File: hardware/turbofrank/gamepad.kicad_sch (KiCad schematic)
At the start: 3 parts, among them J7 D-SUB 9 Male

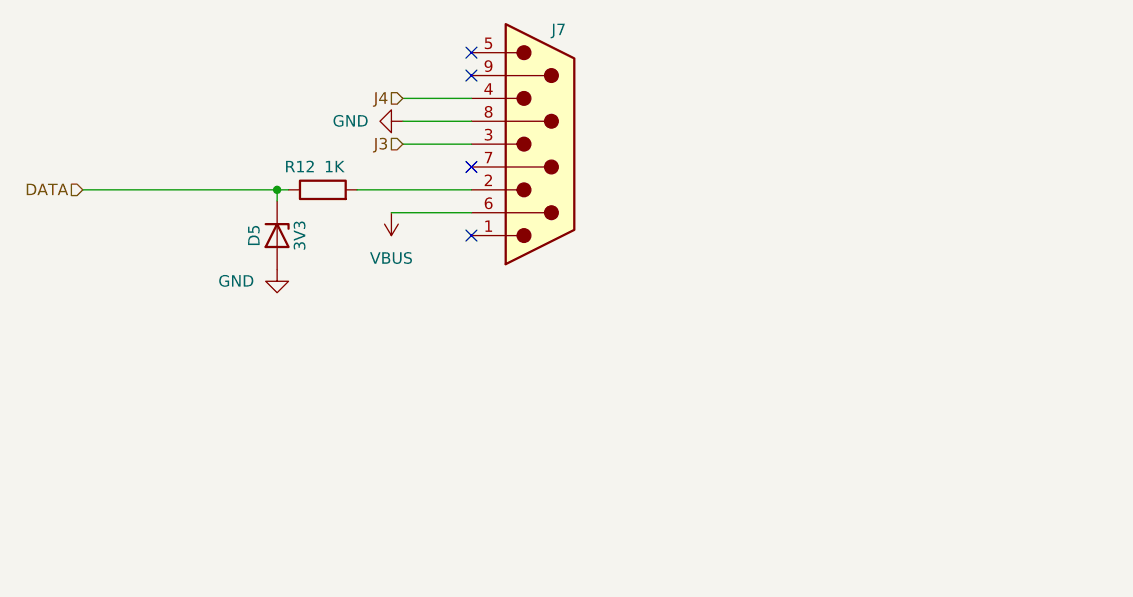
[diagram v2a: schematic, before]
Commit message: TurboFRANK HW 1.05 Release
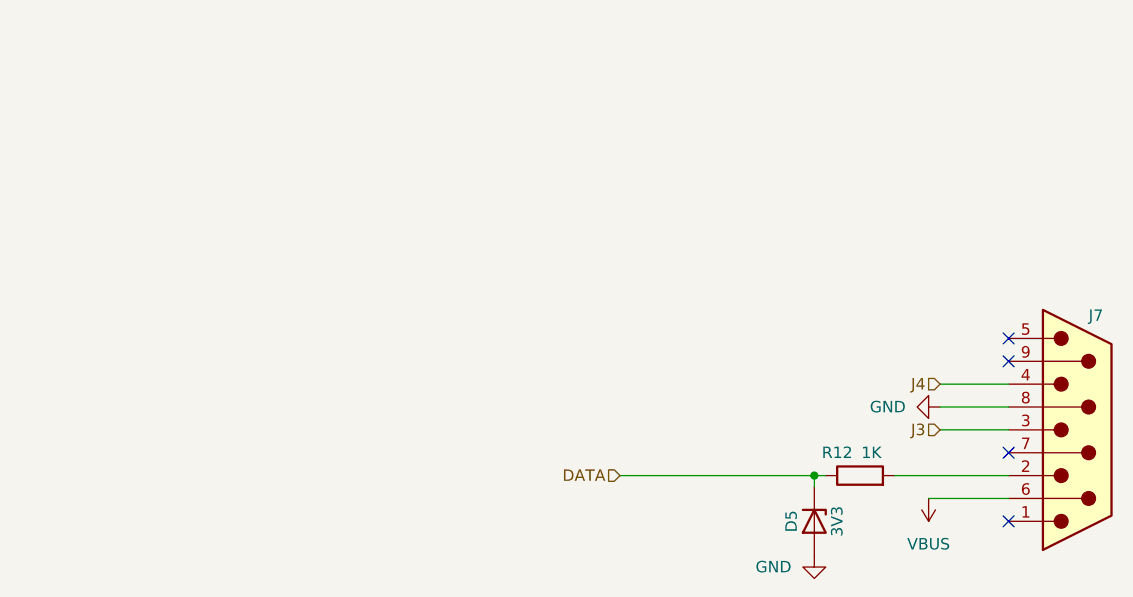
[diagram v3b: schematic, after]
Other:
- moved on the sheet: D5, J7, R12
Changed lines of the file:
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@@
 	)
 	(junction
-		(at 78.74 68.58)
+		(at 138.43 100.33)
 		(diameter 0)
 		(color 0 0 0 0)
 	)
 	(no_connect
-		(at 100.33 55.88)
+		(at 160.02 87.63)
 	)
 	(no_connect
-		(at 100.33 53.34)
+		(at 160.02 85.09)
 	)
 	(no_connect
-		(at 100.33 66.04)
+		(at 160.02 97.79)
 	)
 	(no_connect
-		(at 100.33 73.66)
-	)
-	(wire
-		(pts
-			(xy 92.71 63.5) (xy 100.33 63.5)
-		)
-		(stroke
-			(width 0)
-			(type default)
-		)
-	)
-	(wire
-		(pts
-			(xy 92.71 58.42) (xy 100.33 58.42)
-		)
-		(stroke
-			(width 0)
-			(type default)
-		)
-	)
-	(wire
-		(pts
-			(xy 91.44 71.12) (xy 100.33 71.12)
-		)
-		(stroke
-			(width 0)
-			(type default)
-		)
-	)
-	(wire
-		(pts
-			(xy 78.74 68.58) (xy 78.74 69.85)
-		)
-		(stroke
-			(width 0)
-			(type default)
-		)
-	)
-	(wire
-		(pts
-			(xy 57.15 68.58) (xy 78.74 68.58)
-		)
-		(stroke
-			(width 0)
-			(type default)
-		)
-	)
-	(wire
-		(pts
-			(xy 80.01 68.58) (xy 78.74 68.58)
-		)
-		(stroke
-			(width 0)
-			(type default)
-		)
-	)
-	(wire
-		(pts
-			(xy 92.71 60.96) (xy 100.33 60.96)
-		)
-		(stroke
-			(width 0)
-			(type default)
-		)
-	)
-	(wire
-		(pts
-			(xy 87.63 68.58) (xy 100.33 68.58)
+		(at 160.02 105.41)
+	)
+	(wire
+		(pts
+			(xy 152.4 95.25) (xy 160.02 95.25)
+		)
+		(stroke
+			(width 0)
+			(type default)
+		)
+	)
+	(wire
+		(pts
+			(xy 152.4 90.17) (xy 160.02 90.17)
+		)
+		(stroke
+			(width 0)
+			(type default)
+		)
+	)
+	(wire
+		(pts
+			(xy 151.13 102.87) (xy 160.02 102.87)
+		)
+		(stroke
+			(width 0)
+			(type default)
+		)
+	)
+	(wire
+		(pts
+			(xy 138.43 100.33) (xy 138.43 101.6)
+		)
+		(stroke
+			(width 0)
+			(type default)
+		)
+	)
+	(wire
+		(pts
+			(xy 116.84 100.33) (xy 138.43 100.33)
+		)
+		(stroke
+			(width 0)
+			(type default)
+		)
+	)
+	(wire
+		(pts
+			(xy 139.7 100.33) (xy 138.43 100.33)
+		)
+		(stroke
+			(width 0)
+			(type default)
+		)
+	)
+	(wire
+		(pts
+			(xy 152.4 92.71) (xy 160.02 92.71)
+		)
+		(stroke
+			(width 0)
+			(type default)
+		)
+	)
+	(wire
+		(pts
+			(xy 147.32 100.33) (xy 160.02 100.33)
 		)
 		(stroke
@@
 	(hierarchical_label "J4"
 		(shape input)
-		(at 92.71 58.42 180)
+		(at 152.4 90.17 180)
 		(effects
 			(font
@@
 	(hierarchical_label "J3"
 		(shape input)
-		(at 92.71 63.5 180)
+		(at 152.4 95.25 180)
 		(effects
 			(font
@@
 	(hierarchical_label "DATA"
 		(shape input)
-		(at 57.15 68.58 180)
+		(at 116.84 100.33 180)
 		(effects
 			(font
@@
 	(symbol
 		(lib_id "power:GND")
-		(at 78.74 77.47 0)
+		(at 138.43 109.22 0)
 		(unit 1)
 		(exclude_from_sim no)
@@
 		(dnp no)
 		(property "Reference" "#PWR035"
-			(at 78.74 83.82 0)
+			(at 138.43 115.57 0)
 			(effects
 				(font
@@
 		)
 		(property "Value" "GND"
-			(at 76.2 78.74 0)
+			(at 135.89 110.49 0)
 			(effects
 				(font
@@
 		)
 		(property "Footprint" ""
-			(at 78.74 77.47 0)
+			(at 138.43 109.22 0)
 			(effects
 				(font
@@
 		)
 		(property "Datasheet" ""
-			(at 78.74 77.47 0)
+			(at 138.43 109.22 0)
 			(effects
 				(font
@@
 		)
 		(property "Description" "Power symbol creates a global label with name \"GND\" , ground"
-			(at 78.74 77.47 0)
+			(at 138.43 109.22 0)
 			(effects
 				(font
@@
 	(symbol
 		(lib_id "Device:D_Zener")
-		(at 78.74 73.66 270)
+		(at 138.43 105.41 270)
 		(unit 1)
 		(exclude_from_sim no)
@@
 		(dnp no)
 		(property "Reference" "D5"
-			(at 76.2 73.66 0)
+			(at 135.89 105.41 0)
 			(effects
 				(font
@@
 		)
 		(property "Value" "3V3"
-			(at 81.28 73.66 0)
+			(at 140.97 105.41 0)
 			(effects
 				(font
@@
 		)
 		(property "Footprint" "FRANK:Diode (SOD-323)"
-			(at 78.74 73.66 0)
+			(at 138.43 105.41 0)
 			(effects
 				(font
@@
 		)
 		(property "Datasheet" "https://www.vishay.com/docs/83335/bzx384g.pdf"
-			(at 78.74 73.66 0)
+			(at 138.43 105.41 0)
 			(effects
 				(font
@@
 		)
 		(property "Description" ""
-			(at 78.74 73.66 0)
+			(at 138.43 105.41 0)
 			(effects
 				(font
@@
 		)
 		(property "AliExpress" "https://www.aliexpress.com/item/1005006143480992.html"
-			(at 78.74 73.66 0)
+			(at 138.43 105.41 0)
 			(effects
 				(font
@@
 	(symbol
 		(lib_id "power:VBUS")
-		(at 91.44 71.12 180)
+		(at 151.13 102.87 180)
 		(unit 1)
 		(exclude_from_sim no)
@@
 		(fields_autoplaced yes)
 		(property "Reference" "#PWR034"
-			(at 91.44 67.31 0)
+			(at 151.13 99.06 0)
 			(effects
 				(font
@@
 		)
 		(property "Value" "VBUS"
-			(at 91.44 76.2 0)
+			(at 151.13 107.95 0)
 			(effects
 				(font
@@
 		)
 		(property "Footprint" ""
-			(at 91.44 71.12 0)
+			(at 151.13 102.87 0)
 			(effects
 				(font
@@
 		)
 		(property "Datasheet" ""
-			(at 91.44 71.12 0)
+			(at 151.13 102.87 0)
 			(effects
 				(font
@@
 		)
 		(property "Description" "Power symbol creates a global label with name \"VBUS\""
-			(at 91.44 71.12 0)
+			(at 151.13 102.87 0)
 			(effects
 				(font
@@
 	(symbol
 		(lib_id "FRANK:DB9_Male_Small")
-		(at 107.95 63.5 0)
+		(at 167.64 95.25 0)
 		(unit 1)
 		(exclude_from_sim no)
@@
 		(dnp no)
 		(property "Reference" "J7"
-			(at 109.22 50.8 0)
+			(at 168.91 82.55 0)
 			(effects
 				(font
@@
 		)
 		(property "Value" "D-SUB 9 Male"
-			(at 105.41 48.26 0)
+			(at 165.1 80.01 0)
 			(effects
 				(font
@@
 		)
 		(property "Footprint" "FRANK:D-SUB (9 pin, male, top mount)"
-			(at 107.95 63.5 0)
+			(at 167.64 95.25 0)
 			(effects
 				(font
@@
 		)
 		(property "Datasheet" "https://eu.mouser.com/datasheet/2/578/original-3313093.pdf"
-			(at 107.95 63.5 0)
+			(at 167.64 95.25 0)
 			(effects
 				(font
@@
 		)
 		(property "Description" ""
-			(at 107.95 63.5 0)
+			(at 167.64 95.25 0)
 			(effects
 				(font
@@
 		)
 		(property "AliExpress" "https://www.aliexpress.com/item/4001214300548.html"
-			(at 107.95 63.5 0)
+			(at 167.64 95.25 0)
 			(effects
 				(font
@@
 		(lib_name "GND_1")
 		(lib_id "power:GND")
-		(at 92.71 60.96 270)
+		(at 152.4 92.71 270)
 		(unit 1)
 		(exclude_from_sim no)
@@
 		(fields_autoplaced yes)
 		(property "Reference" "#PWR033"
-			(at 86.36 60.96 0)
+			(at 146.05 92.71 0)
 			(effects
 				(font
@@
 		)
 		(property "Value" "GND"
-			(at 88.9 60.9599 90)
+			(at 148.59 92.7099 90)
 			(effects
 				(font
@@
 		)
 		(property "Footprint" ""
-			(at 92.71 60.96 0)
+			(at 152.4 92.71 0)
 			(effects
 				(font
@@
 		)
 		(property "Datasheet" ""
-			(at 92.71 60.96 0)
+			(at 152.4 92.71 0)
 			(effects
 				(font
@@
 		)
 		(property "Description" "Power symbol creates a global label with name \"GND\" , ground"
-			(at 92.71 60.96 0)
+			(at 152.4 92.71 0)
 			(effects
 				(font
@@
 	(symbol
 		(lib_id "Device:R")
-		(at 83.82 68.58 90)
+		(at 143.51 100.33 90)
 		(unit 1)
 		(exclude_from_sim no)
@@
 		(dnp no)
 		(property "Reference" "R12"
-			(at 81.28 66.04 90)
+			(at 140.97 97.79 90)
 			(effects
 				(font
@@
 		)
 		(property "Value" "1K"
-			(at 85.09 66.04 90)
+			(at 144.78 97.79 90)
 			(effects
 				(font
@@
 		)
 		(property "Footprint" "FRANK:Resistor (0805)"
-			(at 83.82 70.358 90)
+			(at 143.51 102.108 90)
 			(effects
 				(font
@@
 		)
 		(property "Datasheet" "https://www.vishay.com/docs/28952/mcs0402at-mct0603at-mcu0805at-mca1206at.pdf"
-			(at 83.82 68.58 0)
+			(at 143.51 100.33 0)
 			(effects
 				(font
@@
 		)
 		(property "Description" ""
-			(at 83.82 68.58 0)
+			(at 143.51 100.33 0)
 			(effects
 				(font
@@
 		)
 		(property "AliExpress" "https://www.aliexpress.com/item/1005005945735199.html"
-			(at 83.82 68.58 0)
-			(effects
-				(font
+			(at 143.51 100.33 0)
+			(effects
+				(font

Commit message: Bugfixes
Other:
- title: TurboFRANK -> ${NAME}
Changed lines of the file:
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@@
 	(paper "A4")
 	(title_block
-		(title "TurboFRANK")
-		(date "2025-04-04")
+		(title "${NAME}")
+		(date "2025-04-20")
 		(rev "${VERSION}")
 		(company "Mikhail Matveev")
